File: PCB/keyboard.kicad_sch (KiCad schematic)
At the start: 167 parts, among them J1 OLED_128x32, SW1 RotaryEncoder_Switch, U1 Raspberry_Pi_Pico

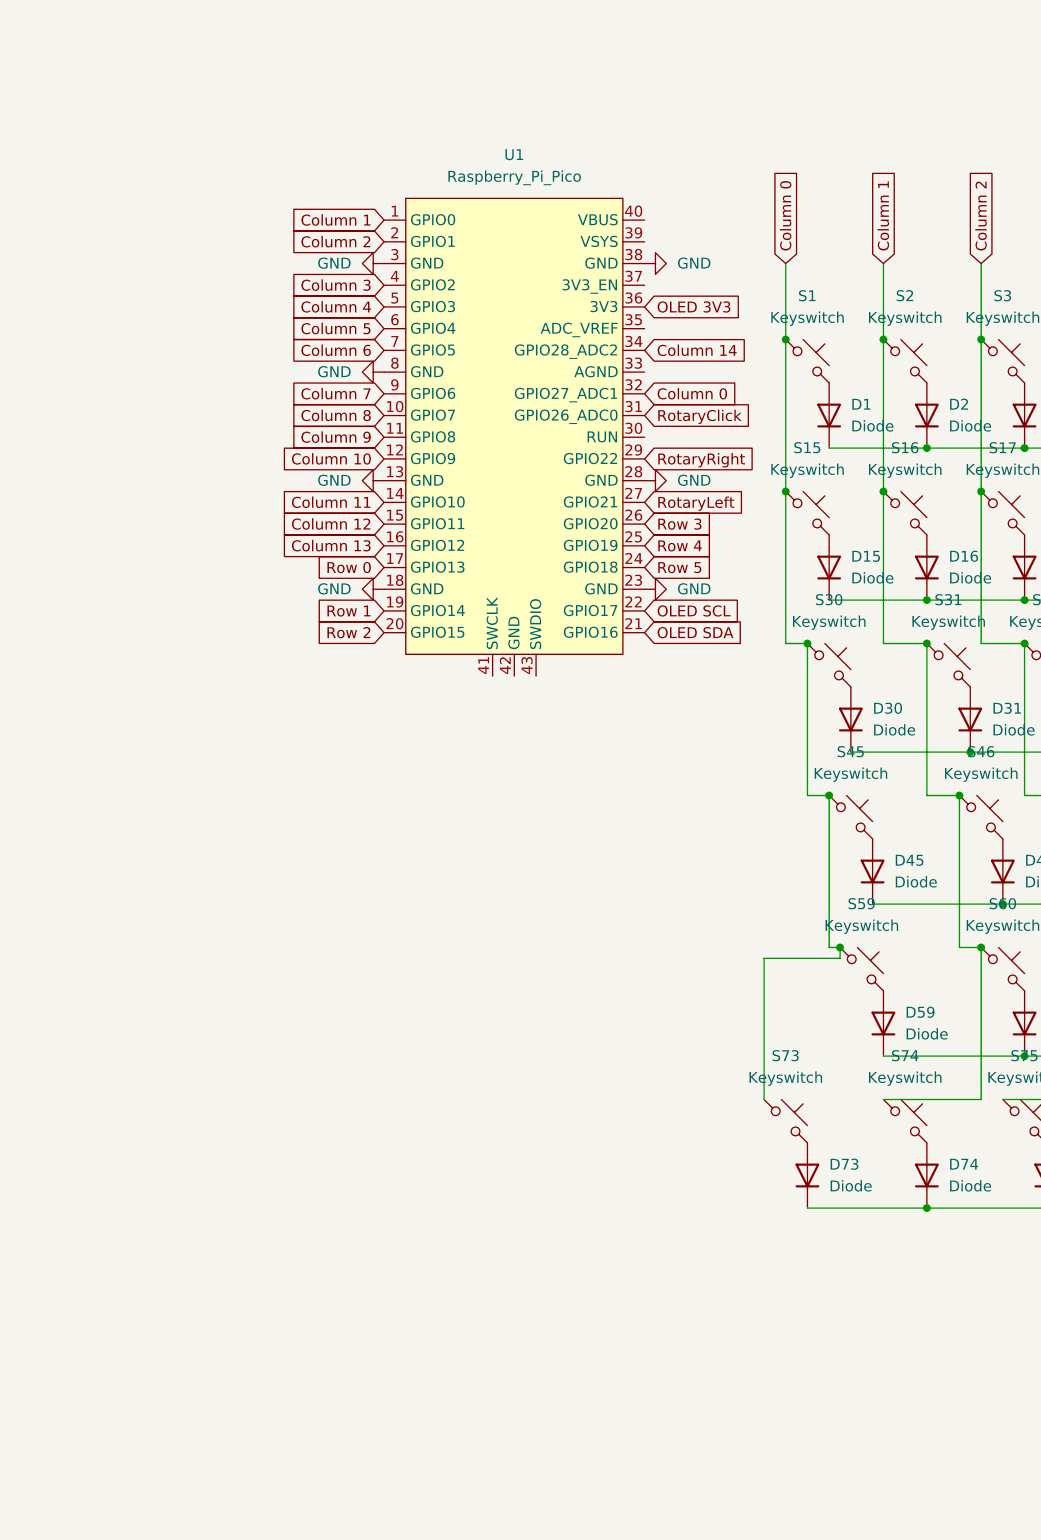
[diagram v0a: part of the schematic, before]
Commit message: Add files via upload
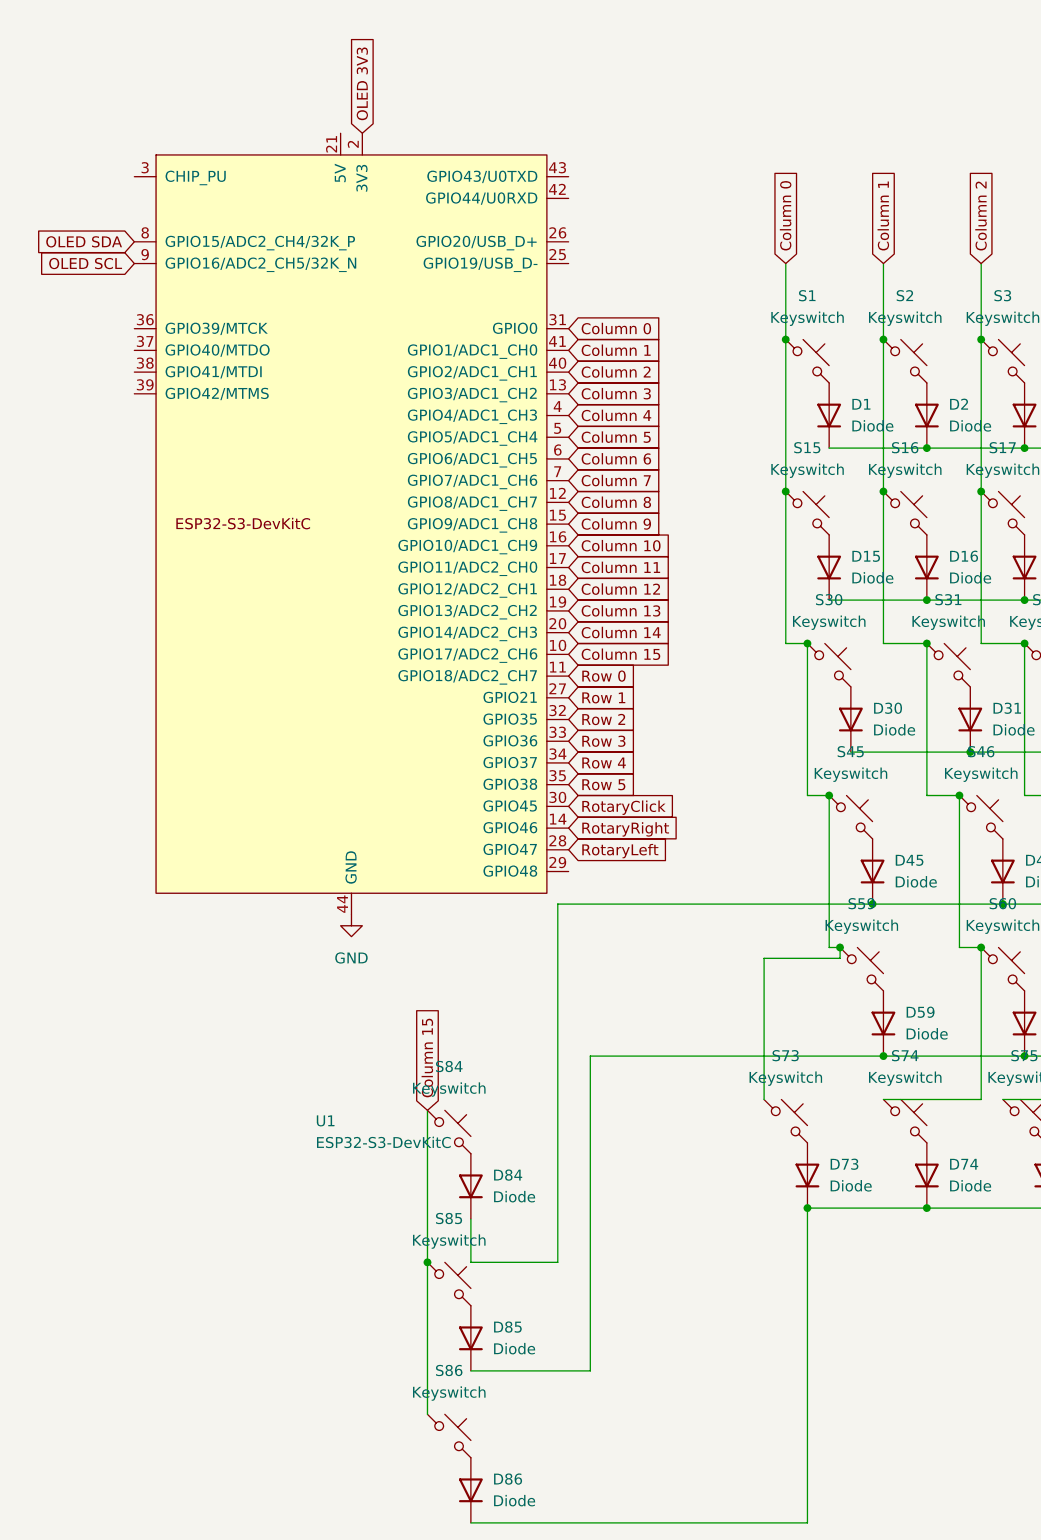
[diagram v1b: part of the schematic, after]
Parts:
- removed U1: Raspberry_Pi_Pico, ScottoKeebs_MCU:Raspberry_Pi_Pico, symbol ScottoKeebs:MCU_Raspberry_Pi_Pico
- added D84, D85, D86: Diode, ScottoKeebs_Components:Diode_DO-35, symbol ScottoKeebs:Placeholder_Diode
- added S84, S85, S86: Keyswitch, ScottoKeebs_Hotswap:Hotswap_MX_1.00u, symbol ScottoKeebs:Placeholder_Keyswitch
- added U1: ESP32-S3-DevKitC, PCM_Espressif:ESP32-S3-DevKitC, symbol PCM_Espressif:ESP32-S3-DevKitC
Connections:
- net Column 0: now also U1.31 (GPIO0)
- net Column 1: now also U1.41 (GPIO1/ADC1_CH0)
- net Column 10: now also U1.16 (GPIO10/ADC1_CH9)
- net Column 11: now also U1.17 (GPIO11/ADC2_CH0)
- net Column 12: now also U1.18 (GPIO12/ADC2_CH1)
- net Column 13: now also U1.19 (GPIO13/ADC2_CH2)
- net Column 14: now also U1.20 (GPIO14/ADC2_CH3)
- net Column 2: now also U1.40 (GPIO2/ADC1_CH1)
- net Column 3: now also U1.13 (GPIO3/ADC1_CH2)
- net Column 4: now also U1.4 (GPIO4/ADC1_CH3)
- net Column 5: now also U1.5 (GPIO5/ADC1_CH4)
- net Column 6: now also U1.6 (GPIO6/ADC1_CH5)
- net Column 7: now also U1.7 (GPIO7/ADC1_CH6)
- net Column 8: now also U1.12 (GPIO8/ADC1_CH7)
- net Column 9: now also U1.15 (GPIO9/ADC1_CH8)
- net GND: now also U1.22 (GND), U1.23 (GND), U1.24 (GND), U1.44 (GND)
- net OLED 3V3: now also U1.1 (3V3), U1.2 (3V3)
- net OLED SCL: now also U1.9 (GPIO16/ADC2_CH5/32K_N)
- net OLED SDA: now also U1.8 (GPIO15/ADC2_CH4/32K_P)
- net RotaryClick: now also U1.30 (GPIO45)
- net RotaryLeft: now also U1.28 (GPIO47)
- net RotaryRight: now also U1.14 (GPIO46)
- net Row 0: now also U1.11 (GPIO18/ADC2_CH7)
- net Row 1: now also U1.27 (GPIO21)
- net Row 2: now also U1.32 (GPIO35)
- net Row 3: now also D84.1 (K), U1.33 (GPIO36)
- net Row 4: now also D85.1 (K), U1.34 (GPIO37)
- net Row 5: now also D86.1 (K), U1.35 (GPIO38)
- new net: D84.2 (A), S84.2
- new net: D85.2 (A), S85.2
- new net: D86.2 (A), S86.2
- new net Column 15: S84.1, S85.1, S86.1, U1.10 (GPIO17/ADC2_CH6)
